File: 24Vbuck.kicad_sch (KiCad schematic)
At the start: 0 parts

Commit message: pm
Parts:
- added C1, C_C1, C_C2, C_C3: C, symbol Device:C
- added R_C1, R_UV1, R_UV2: R, LM5146RGYR:IC_LM5146RGYR, symbol Device:R
- added R_C2, R_FB1, R_FB2: R, symbol Device:R
- added R_RT: 24.9, LM5146RGYR:IC_LM5146RGYR, symbol Device:R
- added U2: LM5146RGYR, LM5146RGYR:IC_LM5146RGYR, symbol LM5146RGYR:LM5146RGYR
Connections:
- new net: C1.2, R_RT.2, U2.2 (RT)
- new net: C_C2.2, R_C1.2, R_FB1.2, R_FB2.1, U2.5 (FB)
- new net: R_UV1.2, R_UV2.2, U2.1 (EN/UVLO)
- new net: C_C1.1, C_C2.1, U2.4 (COMP)
- new net: C_C3.1, R_C2.2
- new net: C_C1.2, R_C1.1
- new net: U2.16 (NC), U2.9 (NC)
- new net 24VPGOOD: U2.10 (PGOOD)
- new net 24Vsync_inn: U2.8 (SYNCIN)
- new net 24Vsync_out: U2.7 (SYNCOUT)
- new net EP: U2.15 (EP), U2.21 (EP)
- new net GND: C1.1, R_FB2.2, R_RT.1, R_UV2.1, U2.6 (AGND)
- new net Vout: R_C2.1, R_FB1.1

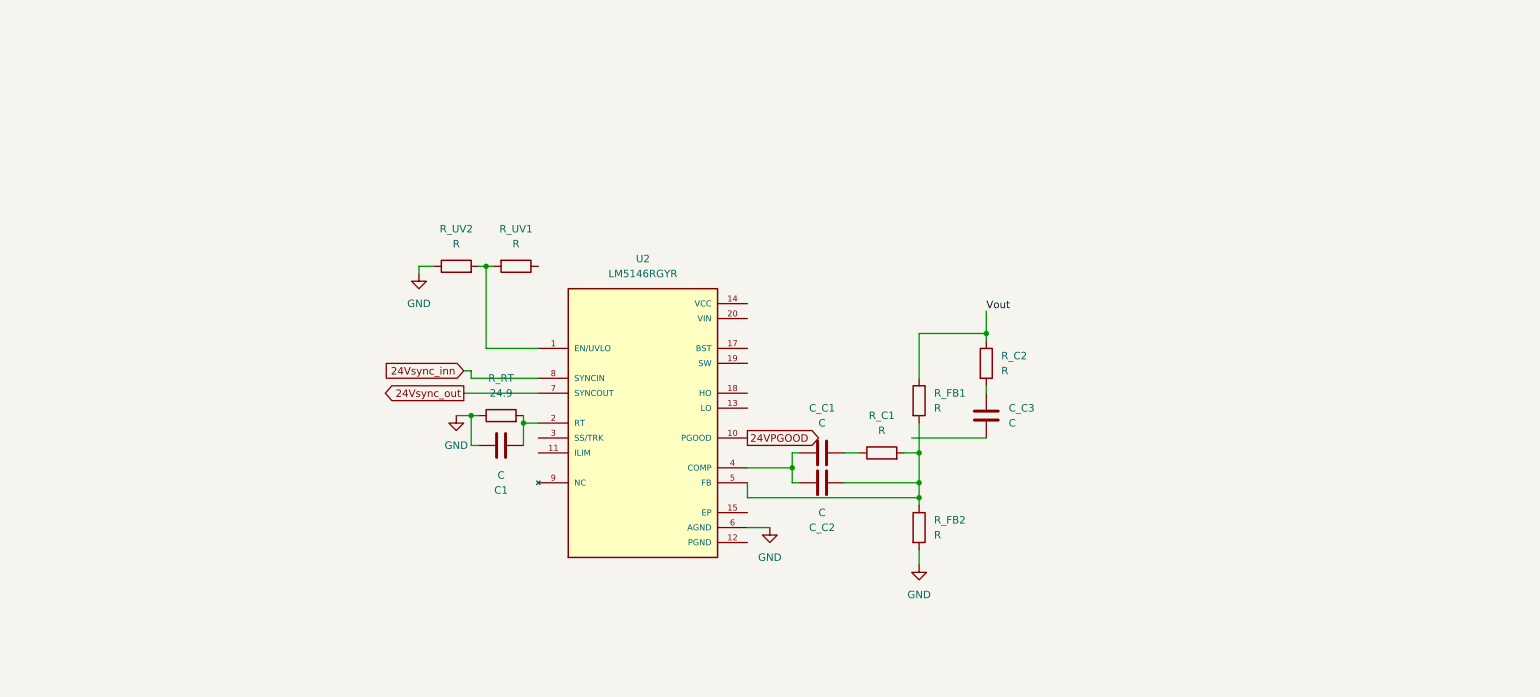
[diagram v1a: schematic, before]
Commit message: LM5146 etter skjema
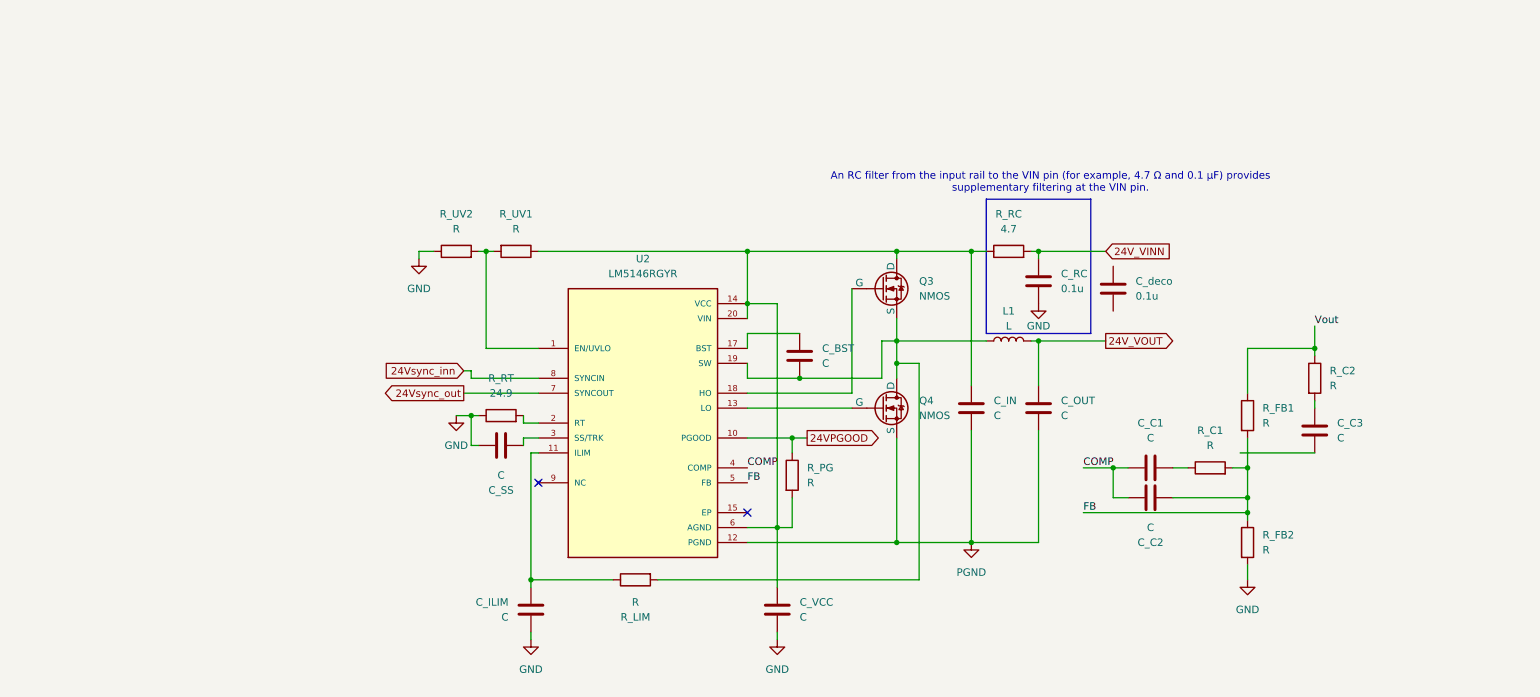
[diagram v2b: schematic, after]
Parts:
- added C_BST, C_ILIM, C_IN, C_OUT, C_VCC: C, symbol Device:C
- added C_RC, C_deco: 0.1u, symbol Device:C
- added L1: L, symbol Device:L
- added Q3, Q4: NMOS, NVMFD5C674NLT1G, symbol Simulation_SPICE:NMOS
- added R_LIM, R_PG: R, symbol Device:R
- added R_RC: 4.7, symbol Device:R
- renumbered C1 to C_SS
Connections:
- net 24VPGOOD: now also R_PG.1
- net GND: now also C_ILIM.2, C_RC.2, C_VCC.2; no longer U2.6 (AGND)
- net at R_RT.2, U2.2 (RT): no longer C_SS.2
- net FB: now reaches C_C2.2, R_C1.2, R_FB1.2, R_FB2.1, U2.5 (FB)
- net COMP: now reaches C_C1.1, C_C2.1, U2.4 (COMP)
- net at R_UV1.1: now also U2.14 (VCC), U2.20 (VIN), U2.6 (AGND), C_IN.1, C_VCC.1, Q3.1 (D), R_PG.2, R_RC.1
- net at U2.11 (ILIM): now also C_ILIM.1, R_LIM.1
- net PGND: now reaches U2.12 (PGND)
- net PGND: now also C_IN.2, C_OUT.2, Q4.3 (S)
- net at U2.13 (LO): now also Q4.2 (G)
- net at U2.17 (BST): now also C_BST.1
- net at U2.18 (HO): now also Q3.2 (G)
- net at U2.19 (SW): now also C_BST.2, L1.1, Q3.3 (S), Q4.1 (D), R_LIM.2
- net at U2.3 (SS/TRK): now also C_SS.2
- new net 24V_VINN: C_RC.1, R_RC.2
- new net 24V_VOUT: C_OUT.1, L1.2
- no-connect marks 0 -> 2
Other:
- note added: "An RC filter from the input rail to the VIN pin (for example, 4.7 Ω and 0.1 µF) provides supplementary filtering at the VIN pin."
- moved on the sheet: C_C1, C_C2, C_C3, R_C1, R_C2, R_FB1, R_FB2, R_UV1, R_UV2

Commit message: Sette opp simuering
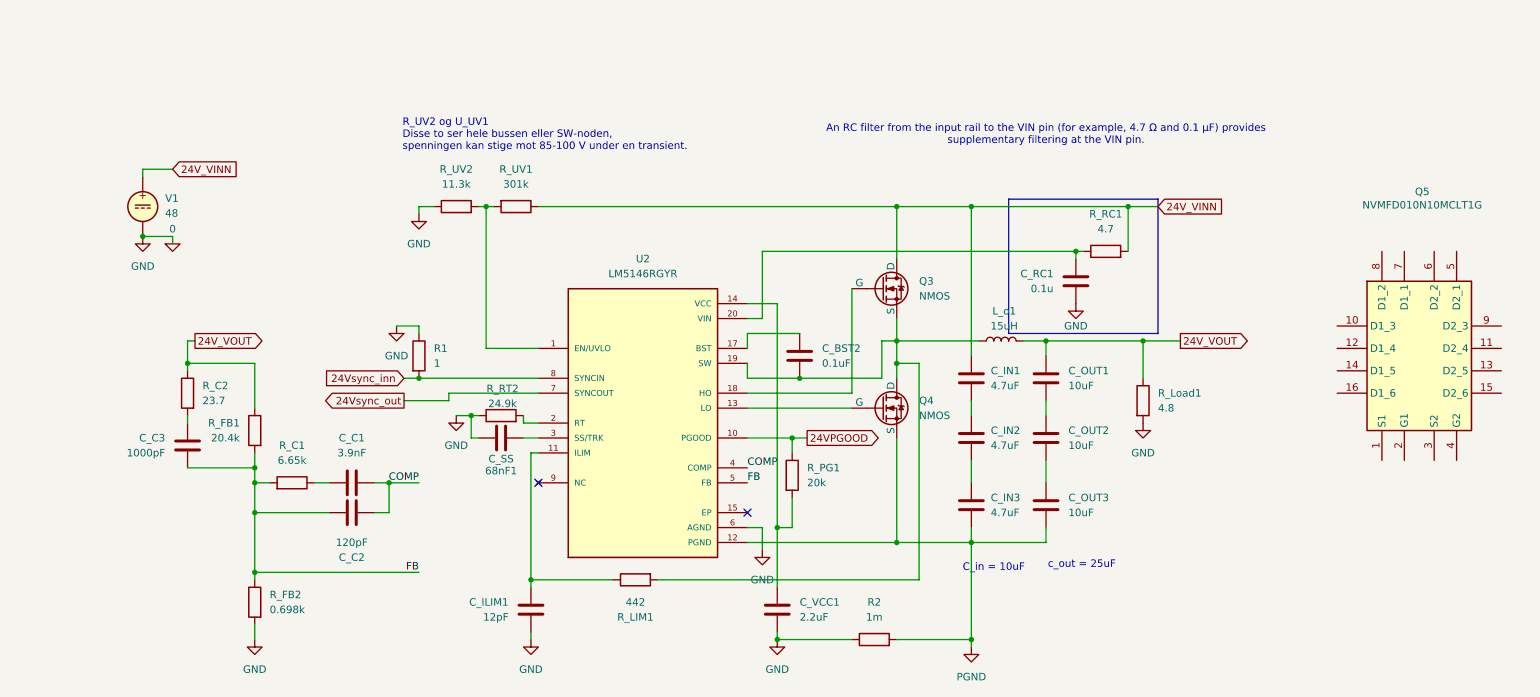
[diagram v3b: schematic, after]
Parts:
- removed C_deco: 0.1u, symbol Device:C
- added C_IN2, C_IN3: 4.7uF, symbol Device:C
- added C_OUT2, C_OUT3: 10uF, symbol Device:C
- added Q5: NVMFD010N10MCLT1G, Marinor:NVMFD5C674NLT1G, symbol Aase:NVMFD010N10MCLT1G
- added R1: 1, symbol Device:R
- added R2: 1m, symbol Device:R
- added R_Load1: 4.8, symbol Device:R
- added V1: 48, Package_SON:WSON-8-1EP_6x5mm_P1.27mm_EP3.4x4mm, symbol Simulation_SPICE:VDC
- 68nF1: renamed from C_SS; value C -> C_SS
- C_BST2: renamed from C_BST; value C -> 0.1uF
- C_C1: value C -> 3.9nF
- C_C2: value C -> 120pF
- C_C3: value C -> 1000pF
- C_ILIM1: renamed from C_ILIM; value C -> 12pF
- C_IN1: renamed from C_IN; value C -> 4.7uF
- C_OUT1: renamed from C_OUT; value C -> 10uF
- C_VCC1: renamed from C_VCC; value C -> 2.2uF
- L_o1: renamed from L1; value L -> 15uH
- R_C1: value R -> 6.65k
- R_C2: value R -> 23.7
- R_FB1: value R -> 20.4k
- R_FB2: value R -> 0.698k
- R_LIM1: renamed from R_LIM; value R -> 442
- R_PG1: renamed from R_PG; value R -> 20k
- R_RT2: renamed from R_RT; value 24.9 -> 24.9k
- R_UV1: value R -> 301k
- R_UV2: value R -> 11.3k
- renumbered C_RC to C_RC1, R_RC to R_RC1
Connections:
- net Vout is gone; now on net 24V_VOUT: R_C2.1, R_FB1.1
- net 24V_VINN: now also C_IN1.1, Q3.1 (D), R_UV1.1, V1.1; no longer C_RC1.1
- net 24V_VOUT: now also R_Load1.1
- net 24Vsync_inn: now also R1.2
- net FB: now also C_C3.2
- net PGND: now also C_IN3.2, C_OUT3.2, R2.2; no longer C_IN1.2, C_OUT1.2
- net at U2.3 (SS/TRK): now also 68nF1.1; no longer 68nF1.2
- net GND renamed 0
- net 0: now also 68nF1.2, U2.6 (AGND), R1.1, R2.1, R_Load1.2, V1.2; no longer 68nF1.1
- new net: C_VCC1.1, R_PG1.2, U2.14 (VCC)
- new net: C_RC1.1, R_RC1.1, U2.20 (VIN)
- new net: C_IN1.2, C_IN2.1
- new net: C_IN2.2, C_IN3.1
- new net: C_OUT1.2, C_OUT2.1
- new net: C_OUT2.2, C_OUT3.1
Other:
- note added: "C_in = 10uF"
- note added: "R_UV2 og U_UV1 Disse to ser hele bussen eller SW-noden, spenningen kan stige mot 85-100 V under en transient."
- note added: "c_out = 25uF"
- moved on the sheet: 68nF1, C_C1, C_C2, C_C3, C_IN1, C_OUT1, C_RC1, L_o1, R_C1, R_C2, R_FB1, R_FB2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

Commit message: valgte verdier, ikke modellnr
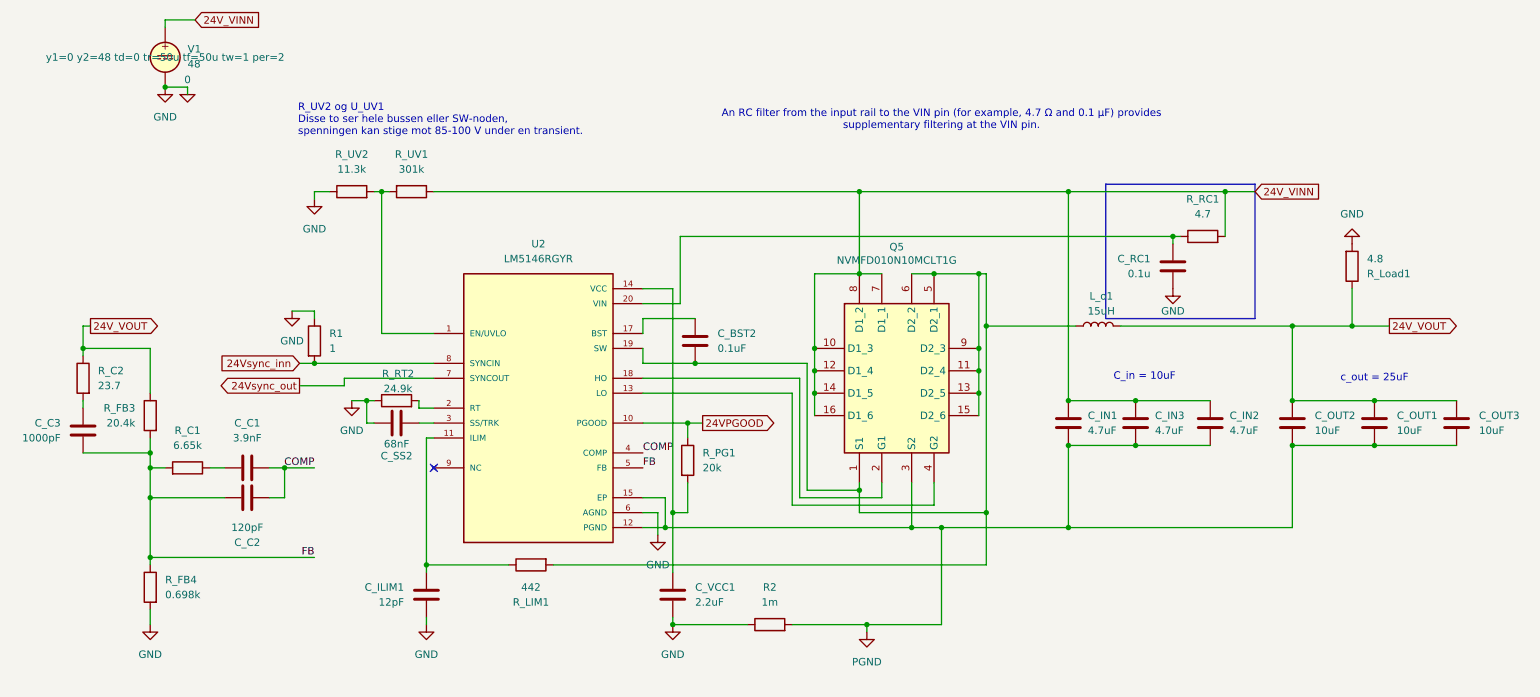
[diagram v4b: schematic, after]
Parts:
- removed 68nF1: C_SS, symbol Device:C
- removed Q3, Q4: NMOS, NVMFD5C674NLT1G, symbol Simulation_SPICE:NMOS
- removed R_FB1: 20.4k, symbol Device:R
- removed R_FB2: 0.698k, symbol Device:R
- added C_SS2: 68nF, symbol Device:C
- added R_FB3: 20.4k, symbol Device:R
- added R_FB4: 0.698k, symbol Device:R
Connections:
- net PGND is gone; now on net EP: C_IN3.2, C_OUT3.2, R2.2, U2.12 (PGND)
- net 0: now also C_SS2.2, R_FB4.2
- net 24V_VINN: now also C_IN2.1, C_IN3.1, Q5.10 (D1_3), Q5.12 (D1_4), Q5.14 (D1_5), Q5.16 (D1_6), Q5.7 (D1_1), Q5.8 (D1_2)
- net 24V_VOUT: now also C_OUT2.1, C_OUT3.1, R_FB3.1
- net EP: now also C_IN1.2, C_IN2.2, C_OUT1.2, C_OUT2.2, Q5.3 (S2)
- net FB: now also R_FB3.2, R_FB4.1
- net at U2.3 (SS/TRK): now also C_SS2.1
- net at C_BST2.2, L_o1.1, R_LIM1.2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: now also Q5.1 (S1), Q5.11 (D2_4), Q5.13 (D2_5), Q5.15 (D2_6), Q5.5 (D2_1), Q5.6 (D2_2), Q5.9 (D2_3)
- net at Q5.2 (G1): now also U2.18 (HO)
- net at Q5.4 (G2): now also U2.13 (LO)
- no-connect marks 2 -> 1
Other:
- moved on the sheet: Q5
